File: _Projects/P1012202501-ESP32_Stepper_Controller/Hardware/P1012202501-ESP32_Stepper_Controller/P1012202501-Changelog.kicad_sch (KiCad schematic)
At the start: 0 parts

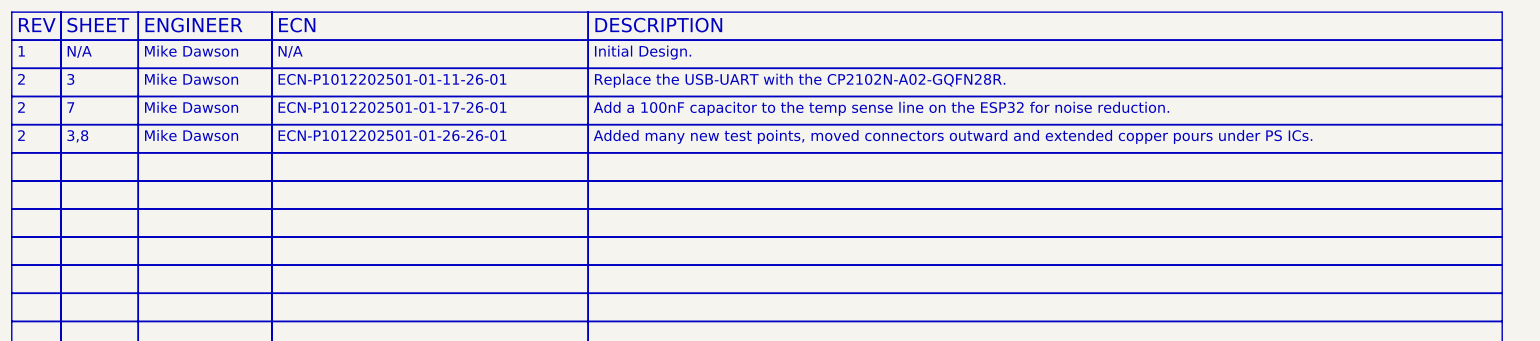
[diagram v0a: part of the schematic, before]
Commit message: Adding new items from recent streams.
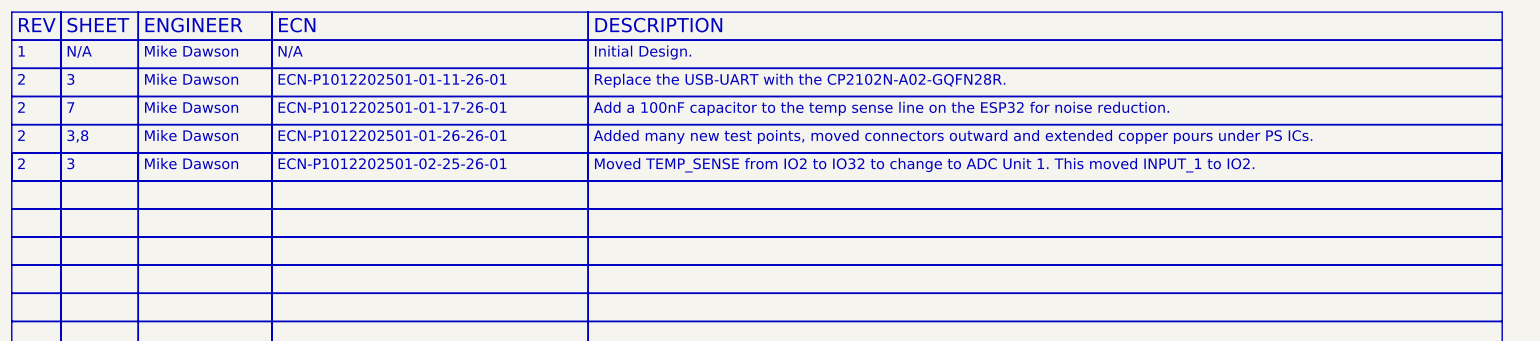
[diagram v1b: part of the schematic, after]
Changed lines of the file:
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@@
+		)
+	)
+	(text_box "2"
+		(exclude_from_sim no)
+		(at 12.7 39.37 0)
+		(size 8.89 5.08)
+		(margins 0.9525 0.9525 0.9525 0.9525)
+		(stroke
+			(width 0.254)
+			(type solid)
+			(color 0 0 0 1)
+		)
+		(fill
+			(type none)
+		)
+		(effects
+			(font
+				(size 1.905 1.905)
+				(color 0 0 0 1)
+			)
+			(justify left top)
 		)
 	)
@@
 		)
 	)
+	(text_box "ECN-P1012202501-02-25-26-01"
+		(exclude_from_sim no)
+		(at 59.69 39.37 0)
+		(size 57.15 5.08)
+		(margins 0.9525 0.9525 0.9525 0.9525)
+		(stroke
+			(width 0.254)
+			(type solid)
+			(color 0 0 0 1)
+		)
+		(fill
+			(type none)
+		)
+		(effects
+			(font
+				(size 1.905 1.905)
+				(color 0 0 0 1)
+			)
+			(justify left top)
+		)
+	)
 	(text_box "3,8"
 		(exclude_from_sim no)
@@
 		)
 	)
+	(text_box "Moved TEMP_SENSE from IO2 to IO32 to change to ADC Unit 1. This moved INPUT_1 to IO2.\n"
+		(exclude_from_sim no)
+		(at 116.84 39.37 0)
+		(size 165.1 5.08)
+		(margins 0.9525 0.9525 0.9525 0.9525)
+		(stroke
+			(width 0.254)
+			(type solid)
+			(color 0 0 0 1)
+		)
+		(fill
+			(type none)
+		)
+		(effects
+			(font
+				(size 1.905 1.905)
+				(color 0 0 0 1)
+			)
+			(justify left top)
+		)
+	)
 	(text_box ""
 		(exclude_from_sim no)
@@
 		)
 	)
+	(text_box "3"
+		(exclude_from_sim no)
+		(at 21.59 39.37 0)
+		(size 13.97 5.08)
+		(margins 0.9525 0.9525 0.9525 0.9525)
+		(stroke
+			(width 0.254)
+			(type solid)
+			(color 0 0 0 1)
+		)
+		(fill
+			(type none)
+		)
+		(effects
+			(font
+				(size 1.905 1.905)
+				(color 0 0 0 1)
+			)
+			(justify left top)
+		)
+	)
 	(text_box ""
 		(exclude_from_sim no)
@@
 		(margins 0.9525 0.9525 0.9525 0.9525)
 		(stroke
+			(width 0.254)
+			(type solid)
+			(color 0 0 0 1)
+		)
+		(fill
+			(type none)
+		)
+		(effects
+			(font
+				(size 1.905 1.905)
+				(color 0 0 0 1)
+			)
+			(justify left top)
+		)
+	)
+	(text_box "Mike Dawson"
+		(exclude_from_sim no)
+		(at 35.56 39.37 0)
+		(size 24.13 5.08)
+		(margins 0.9525 0.9525 0.9525 0.9525)
+		(stroke
